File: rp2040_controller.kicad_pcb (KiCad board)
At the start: 4 copper layers, 19 x 31.5 mm, 34 parts, among them J1 FFC connector, J2 Right, J3 Bottom pin pads, J4 Left, J5 Conn_01x04, J6 Molex Pico Ezmate 1x04 or 1x06, U1 RP2040, U2 AP2112K-3.3TRG1, U3 W25Q64JV, Y1 XYDBPCNANF-12MHZ

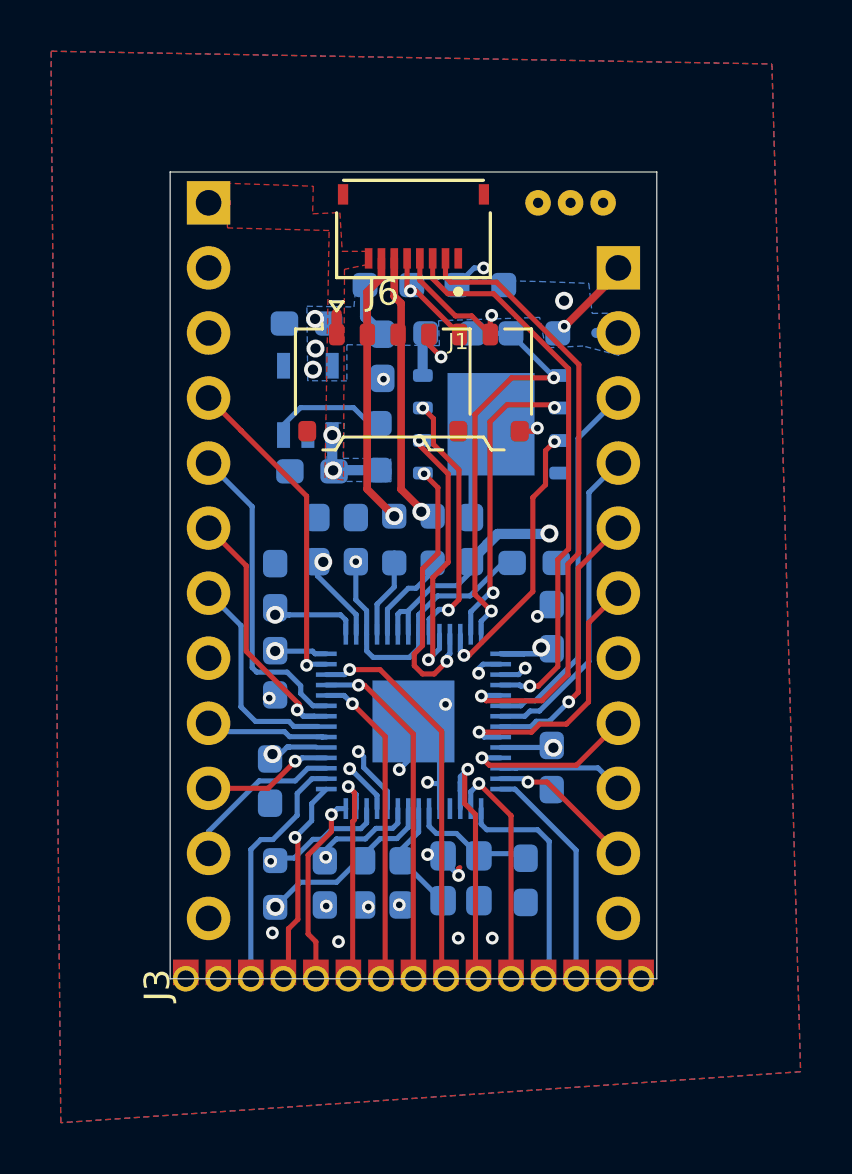
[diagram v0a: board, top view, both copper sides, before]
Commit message: v0.2
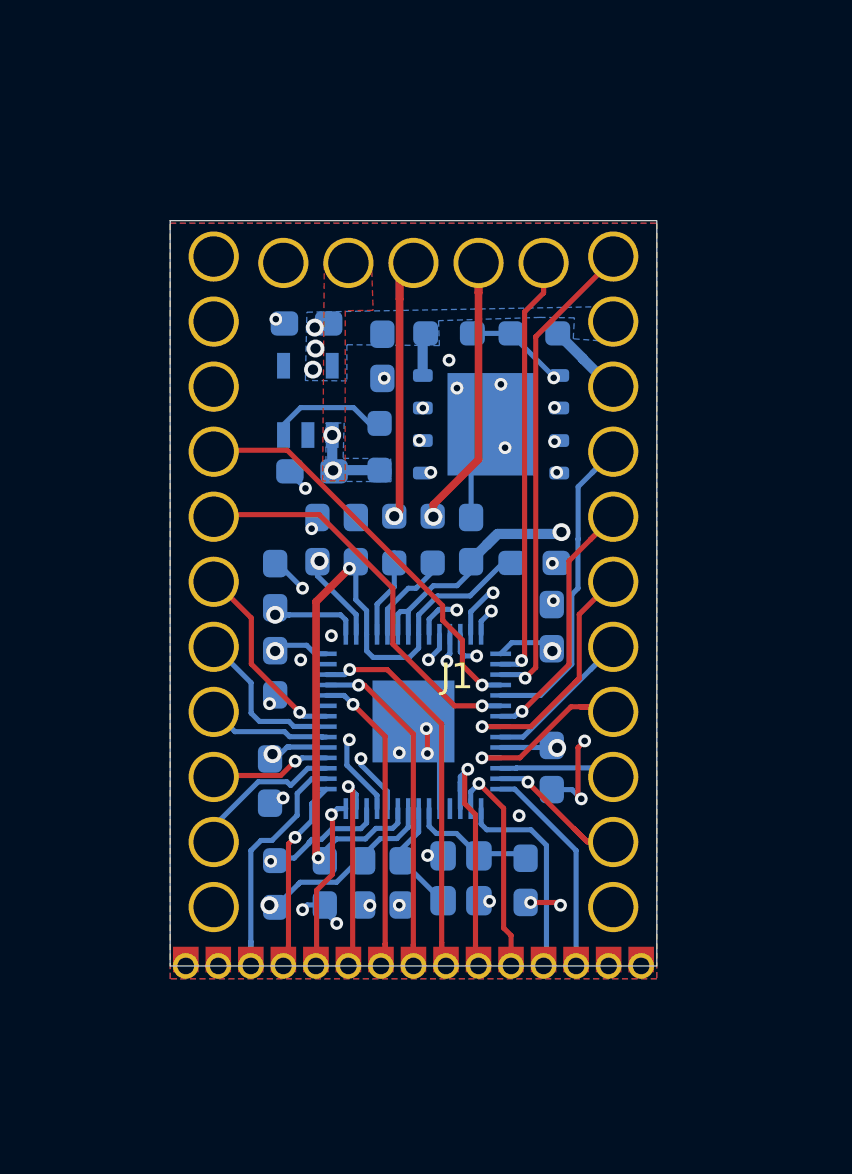
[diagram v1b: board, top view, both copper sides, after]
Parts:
- removed J2: Right, ec_parts:Right_PinHeader_1x11_P2.54mm_Vertical
- removed J3: Bottom pin pads, ec_parts:ec_pad_1x15_P1.27mm
- removed J4: Left, ec_parts:Left_PinHeader_1x12_P2.54mm_Vertical
- removed J5: Conn_01x04, ec_parts:TestPinHeader_1x03_P1.27mm_Vertical
- removed J6: Molex Pico Ezmate 1x04 or 1x06, ec_parts:Molex_Pico-EZmate_1.2mm_04_or_06
- removed R2, R6: 27, Resistor_SMD_AKL:R_0603_1608Metric_Pad0.98x0.95mm_HandSolder
- J1: value FFC connector -> rp2040_controller; footprint ec_parts:HRS_FH34SRJ-08S-0.5SH(50) -> ec_parts:rp2040_controller
- moved J1 14.5 mm to (100.0, 85.2), turned to 0 degrees
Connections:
- J1 pad 1: GND -> /SWCLK
- J1 pad 2: /GPIO3 -> /VSYS
- J1 pad 3: /GPIO2 -> /USB_N
- J1 pad 4: /GPIO1 -> /USB_P
- J1 pad 6: /USB_P -> /GPIO1
- J1 pad 7: /USB_N -> +3V3
- J1 pad 8: /VSYS -> /USB_BOOT
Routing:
- net /GPIO29/ADC3: track 12.8 -> 0.00 mm, vias 1 -> 0
- net /GPIO25: track 12.4 -> 0.00 mm
- net /GPIO3: track 24.3 -> 13.7 mm, vias 1 -> 0
- net /SWCLK: track 32.4 -> 23.5 mm
- net /GPIO2: track 21.9 -> 15.9 mm
- net +3V3: track 39.5 -> 33.9 mm, vias 12 -> 11
- net /GPIO1: track 24.1 -> 18.8 mm, vias 3 -> 1
- net GND: track 9.96 -> 15.2 mm, vias 17 -> 30
- net /RUN: track 28.6 -> 23.9 mm
- net /SWDIO: track 30.7 -> 26.4 mm
- net /GPIO7: track 10.4 -> 7.38 mm, vias 1 -> 0
- net /GPIO24: track 10.5 -> 7.65 mm
- net /GPIO0: track 21.1 -> 18.2 mm, vias 2 -> 1
- net /GPIO8: track 6.85 -> 9.33 mm
- net /GPIO23: track 8.31 -> 6.09 mm
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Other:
- board size 19 x 31.5 mm -> 19 x 29.1 mm

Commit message: v0.3
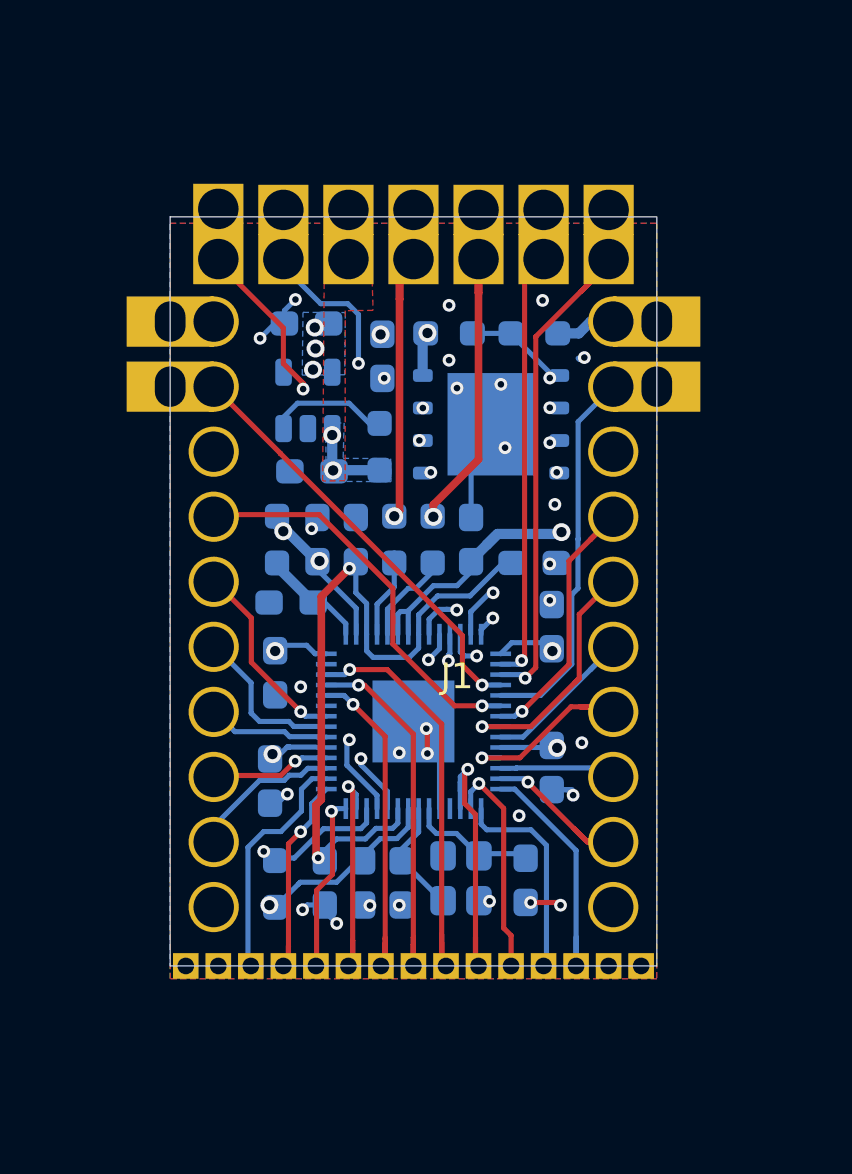
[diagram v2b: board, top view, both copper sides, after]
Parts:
- added R2: 400, Resistor_SMD_AKL:R_0603_1608Metric_Pad0.98x0.95mm_HandSolder, B.Cu at (94.7, 82.9)
- U2: value AP2112K-3.3TRG1 -> AP2112K-3.3; footprint ap2112:AP2112K-3.3TRG1 -> Package_TO_SOT_SMD_AKL:SOT-23-5
- moved C8 0.91 mm to (95.2, 85.3), turned to 180 degrees
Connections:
- C8 pad 1: +3V3 -> /AVDD
- J1 pad 39: /GPIO2 -> GND
- J1 pad 40: /RUN -> /GPIO2
- J1 pad 41: GND -> /RUN
- J1 pad 7: +3V3 -> /USB_BOOT
- J1 pad 8: /USB_BOOT -> /GPIO3
- J1 pad 9: /GPIO3 -> +3V3
- U1 pad 43: +3V3 -> /AVDD
- Y1 pad 2: GND -> unconnected-(Y1-Pad2)
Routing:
- net /AVDD: track 0.00 -> 4.03 mm
- net GND: track 15.2 -> 12.6 mm
- net /GPIO0: track 18.2 -> 15.9 mm
- net /RUN: track 23.9 -> 25.9 mm
- net +3V3: track 33.9 -> 32.1 mm, vias 11 -> 13
- net /GPIO1: track 18.8 -> 20.3 mm
- net /SWDIO: track 26.4 -> 25.0 mm, vias 1 -> 2
- net /GPIO19: track 10.4 -> 9.18 mm
- net /GPIO3: track 13.7 -> 14.8 mm
- net /USB_BOOT: track 3.36 -> 2.36 mm
- net /GPIO28/ADC2: track 15.7 -> 16.5 mm
- net /GPIO2: track 15.9 -> 16.7 mm
- net /GPIO11: track 8.45 -> 9.20 mm
- net /GPIO27/ADC1: track 13.8 -> 14.6 mm
- net /SWCLK: track 23.5 -> 24.2 mm, vias 1 -> 2
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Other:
- board size 19 x 29.1 mm -> 19 x 29.2 mm

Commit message: temp
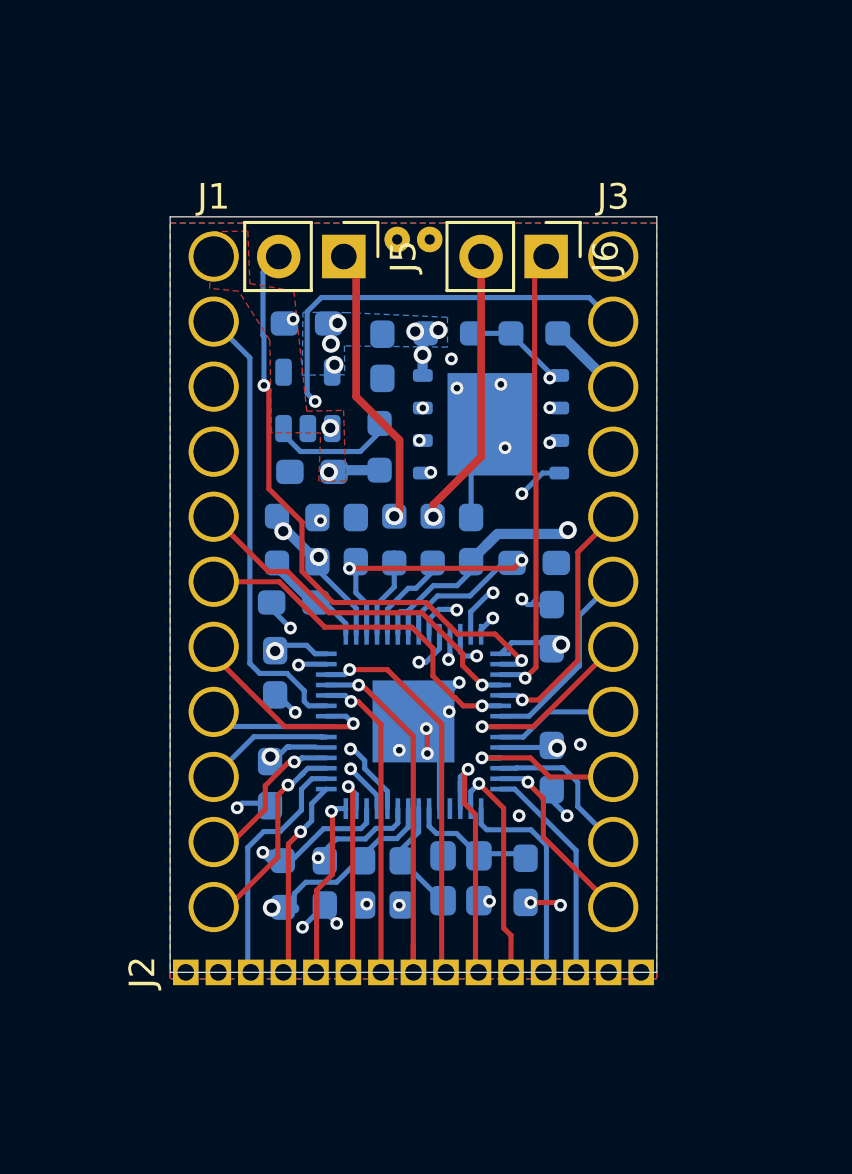
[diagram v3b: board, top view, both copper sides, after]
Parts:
- added J2: Conn_01x15, ec_parts:PinHeader_1x15_P1.27mm_Vertical, F.Cu at (91.1, 99.8)
- added J3: Conn_01x12, ec_parts:PinHeader_1x12_P2.54mm_Vertical, F.Cu at (107.8, 71.8)
- added J4: Conn_01x05, ec_parts:TestPinHeader_1x03_P1.27mm_Vertical, F.Cu at (100.0, 71.1)
- added J5: Conn_01x02, Connector_PinHeader_2.54mm:PinHeader_1x02_P2.54mm_Vertical, F.Cu at (97.3, 71.8)
- added J6: Conn_01x02, Connector_PinHeader_2.54mm:PinHeader_1x02_P2.54mm_Vertical, F.Cu at (105.2, 71.8)
- J1: value rp2040_controller -> Conn_01x12; footprint ec_parts:rp2040_controller -> ec_parts:PinHeader_1x12_P2.54mm_Vertical
- moved J1 15.5 mm to (92.2, 71.8)
- moved R1 0.30 mm to (94.9, 96.3)
- moved C5 0.10 mm to (94.4, 92.4)
- moved C8 0.10 mm to (95.3, 85.3)
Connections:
- J1 pad 1: /SWCLK -> /VSYS
- J1 pad 10: /GPIO5 -> /GPIO21
- J1 pad 11: /GPIO6 -> /GPIO20
- J1 pad 2: /VSYS -> /GPIO25
- J1 pad 3: /USB_N -> /RUN
- J1 pad 4: /USB_P -> GND
- J1 pad 5: /GPIO0 -> /GP_2/I2C_1_SDA/SPI_0_SCK
- J1 pad 6: /GPIO1 -> /GP_4/I2C_0_SDA/SPI_0_RX
- J1 pad 7: /USB_BOOT -> /GPIO24
- J1 pad 8: /GPIO3 -> /GPIO23
- J1 pad 9: +3V3 -> /GPIO22
- U1 pad 2: /GPIO0 -> /GPIO0/I2C0_SDA
- U1 pad 3: /GPIO1 -> /GPIO1/I2C0_SCL
- U1 pad 4: /GPIO2 -> /GP_2/I2C_1_SDA/SPI_0_SCK
- U1 pad 5: /GPIO3 -> /GP_3/I2C_1_SCL/SPI_0_TX 
- U1 pad 6: /GPIO4 -> /GP_4/I2C_0_SDA/SPI_0_RX
- U1 pad 7: /GPIO5 -> /GP_5/I2C_0_SCL/SPI_0_CS
- U1 pad 8: /GPIO6 -> /GP_6/I2C_1_SDA/SPI_0_SCK
- U1 pad 9: /GPIO7 -> /GP_7/I2C_1_SCL/SPI_0_TX
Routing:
- net /GPIO29/ADC3: track 0.00 -> 29.2 mm, vias 0 -> 2
- net /GPIO0/I2C0_SDA: track 0.00 -> 24.1 mm, vias 0 -> 2
- net /GPIO1: track 20.3 -> 0.00 mm, vias 1 -> 0
- net /GPIO25: track 0.00 -> 17.8 mm
- net /GPIO1/I2C0_SCL: track 0.00 -> 17.2 mm, vias 0 -> 1
- net /GPIO2: track 16.7 -> 0.00 mm, vias 1 -> 0
- net /GPIO0: track 15.9 -> 0.00 mm, vias 1 -> 0
- net /GPIO4: track 15.5 -> 0.00 mm, vias 1 -> 0
- net /GPIO3: track 14.8 -> 0.00 mm
- net /GP_2/I2C_1_SDA/SPI_0_SCK: track 0.00 -> 14.2 mm, vias 0 -> 1
- net /GP_4/I2C_0_SDA/SPI_0_RX: track 0.00 -> 13.8 mm, vias 0 -> 1
- net /GPIO5: track 11.8 -> 0.00 mm, vias 1 -> 0
- net /GP_3/I2C_1_SCL/SPI_0_TX : track 0.00 -> 9.91 mm, vias 0 -> 1
- net /GPIO6: track 9.89 -> 0.00 mm, vias 1 -> 0
- net /GP_5/I2C_0_SCL/SPI_0_CS: track 0.00 -> 7.72 mm
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- removed copper zone on B.Cu, net /VSYS
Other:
- board size 19 x 29.2 mm -> 19 x 29.5 mm
